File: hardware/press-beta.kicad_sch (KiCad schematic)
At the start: 28 parts, among them SW1 SW_Push_45deg, SW10 SW_Push_45deg, SW11 SW_Push_45deg, SW12 SW_Push_45deg, SW13 SW_Push_45deg, SW14 SW_Push_45deg, SW15 SW_Push_45deg, SW16 SW_Push_45deg, SW17 SW_Push_45deg, SW18 SW_Push_45deg, SW19 SW_Push_45deg, SW2 SW_Push_45deg, SW20 SW_Push_45deg, SW21 SW_Push_45deg, SW22 SW_Push_45deg, SW23 SW_Push_45deg, SW24 SW_Push_45deg, SW3 SW_Push_45deg, SW4 SW_Push_45deg, SW5 SW_Push_45deg, SW6 SW_Push_45deg, SW7 SW_Push_45deg, SW8 SW_Push_45deg, SW9 SW_Push_45deg, U1 Pico

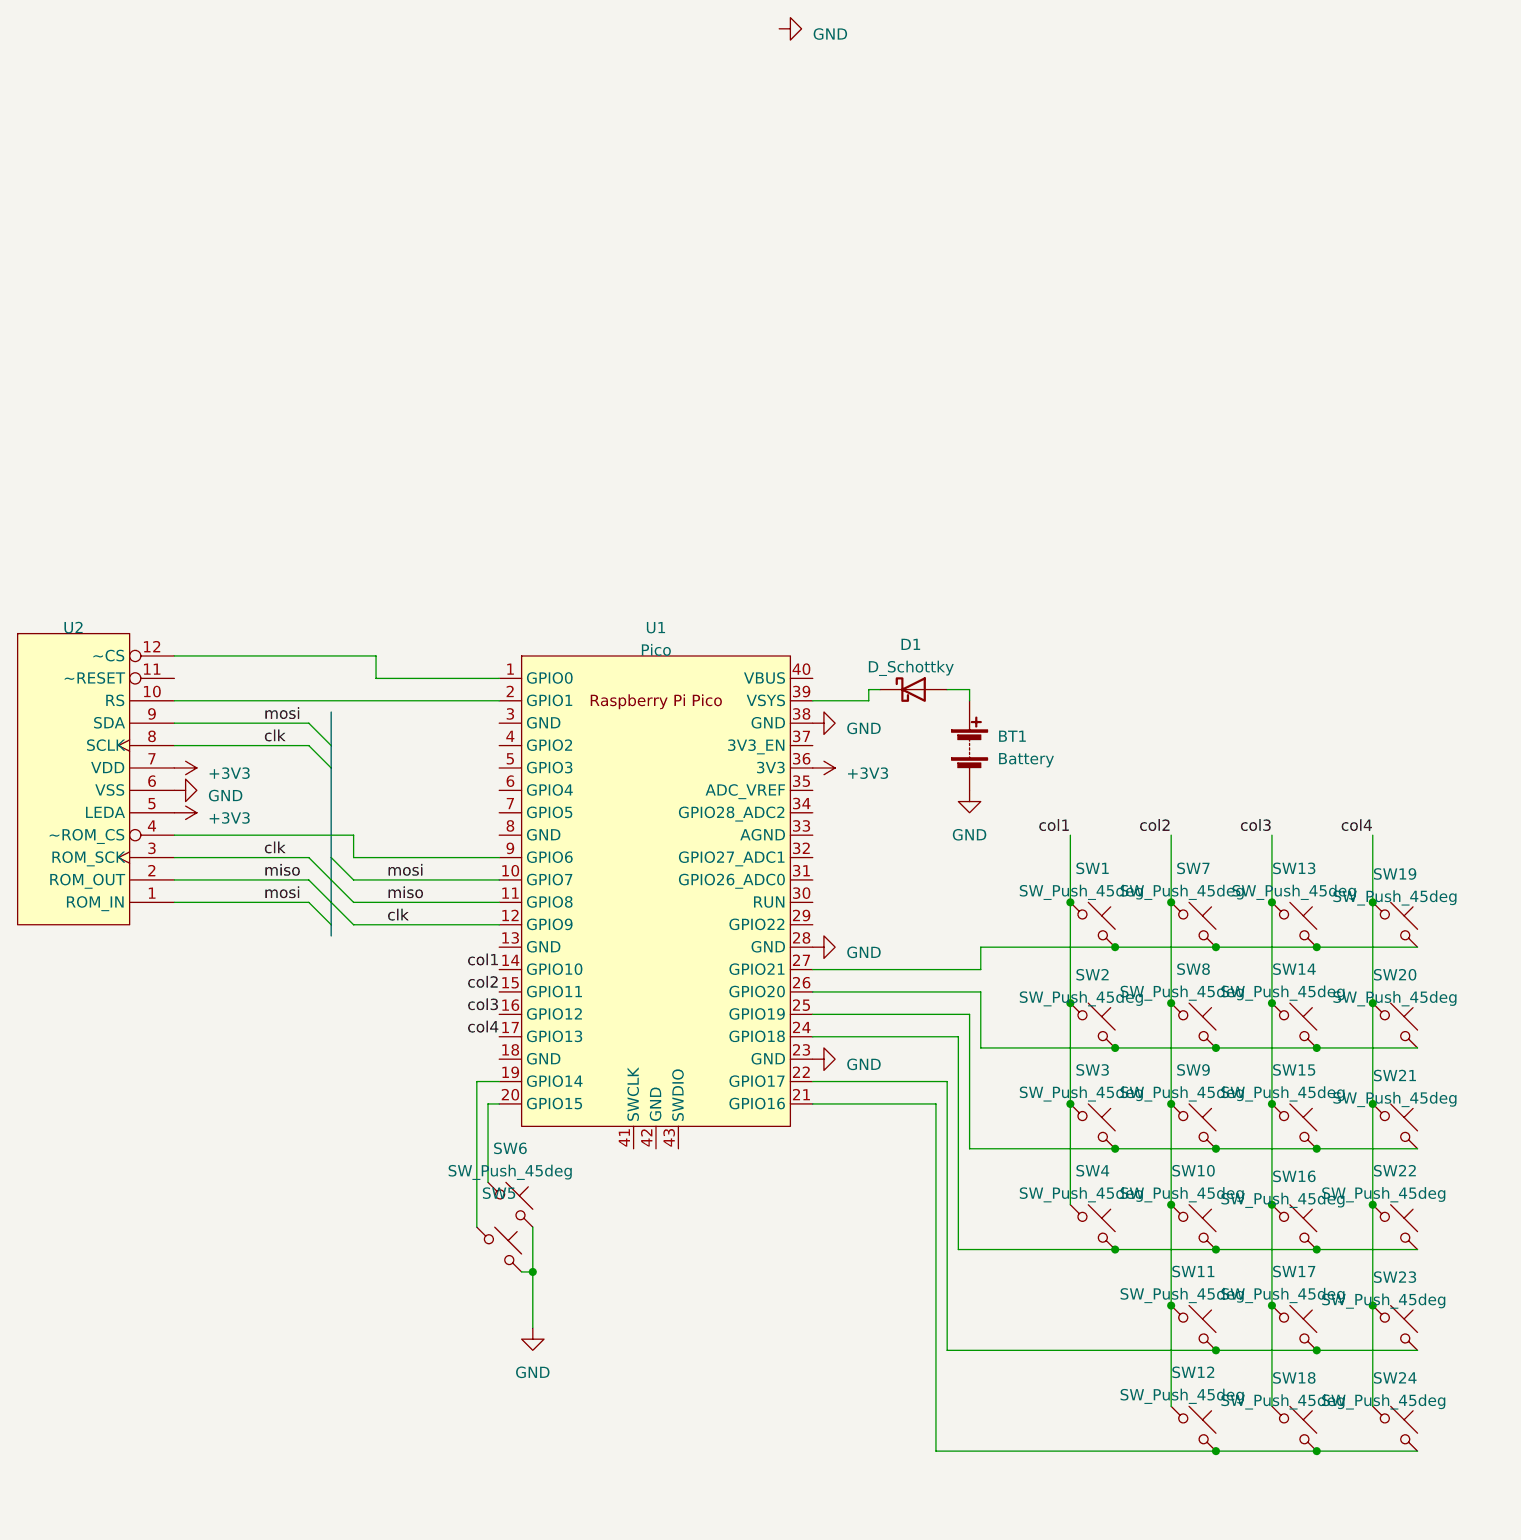
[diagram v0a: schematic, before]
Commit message: pcb mod
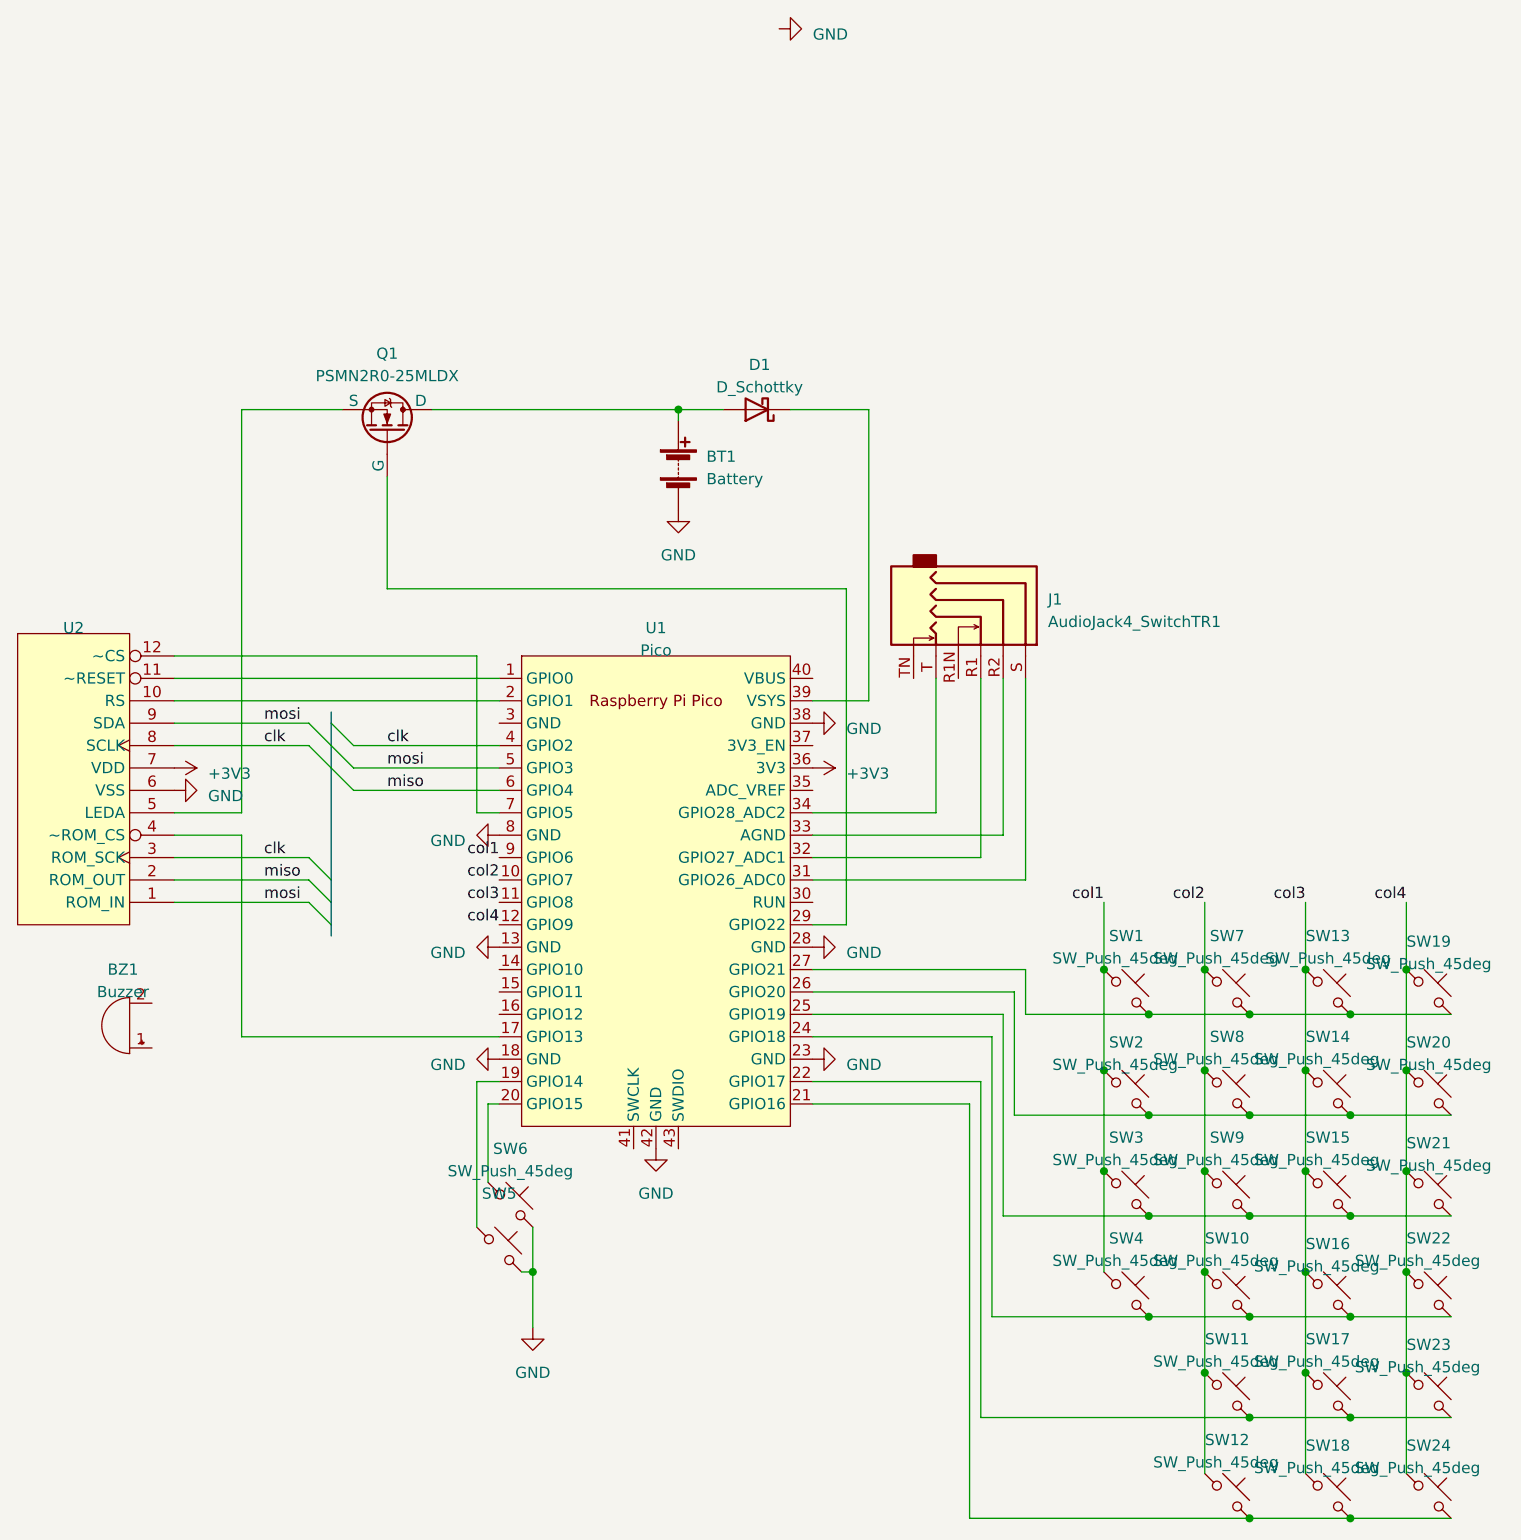
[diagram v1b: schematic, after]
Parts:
- added BZ1: Buzzer, symbol Device:Buzzer
- added J1: AudioJack4_SwitchTR1, Connector_Audio:Jack_3.5mm_PJ311_Horizontal, symbol Connector_Audio:AudioJack4_SwitchTR1
- added Q1: PSMN2R0-25MLDX, Package_TO_SOT_SMD:LFPAK33, symbol Simulation_SPICE:NMOS
- BT1: footprint Battery:BatteryHolder_TruPower_BH-331P_3xAA -> Connector_Wire:SolderWire-0.75sqmm_1x02_P4.8mm_D1.25mm_OD2.3mm
- U2: footprint Library:LCD -> Library:LCD_nopost
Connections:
- net +3V3: no longer U2.5 (LEDA)
- net GND: now also U1.13 (GND), U1.18 (GND), U1.42 (GND), U1.8 (GND)
- net clk: now also U1.4 (GPIO2); no longer U1.12 (GPIO9)
- net col1: now also U1.9 (GPIO6); no longer U1.14 (GPIO10)
- net col2: now also U1.10 (GPIO7); no longer U1.15 (GPIO11)
- net col3: now also U1.11 (GPIO8); no longer U1.16 (GPIO12)
- net col4: now also U1.12 (GPIO9); no longer U1.17 (GPIO13)
- net miso: now also U1.6 (GPIO4); no longer U1.11 (GPIO8)
- net mosi: now also U1.5 (GPIO3); no longer U1.10 (GPIO7)
- net at BT1.1 (+), D1.2 (A): now also Q1.1 (D)
- net at U1.1 (GPIO0): now also U2.11 (~RESET); no longer U2.12 (~CS)
- net at U1.29 (GPIO22): now also Q1.2 (G)
- net at U1.31 (GPIO26_ADC0): now also J1.S
- net at U1.32 (GPIO27_ADC1): now also J1.R1
- net at U1.33 (AGND): now also J1.R2
- net at U1.34 (GPIO28_ADC2): now also J1.T
- net at U1.7 (GPIO5): now also U2.12 (~CS)
- net at U2.4 (~ROM_CS): now also U1.17 (GPIO13); no longer U1.9 (GPIO6)
- new net: Q1.3 (S), U2.5 (LEDA)
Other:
- moved on the sheet: BT1, D1, SW1, SW10, SW11, SW12, SW13, SW14, SW15, SW16, SW17, SW18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
